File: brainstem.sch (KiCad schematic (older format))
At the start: 2 parts

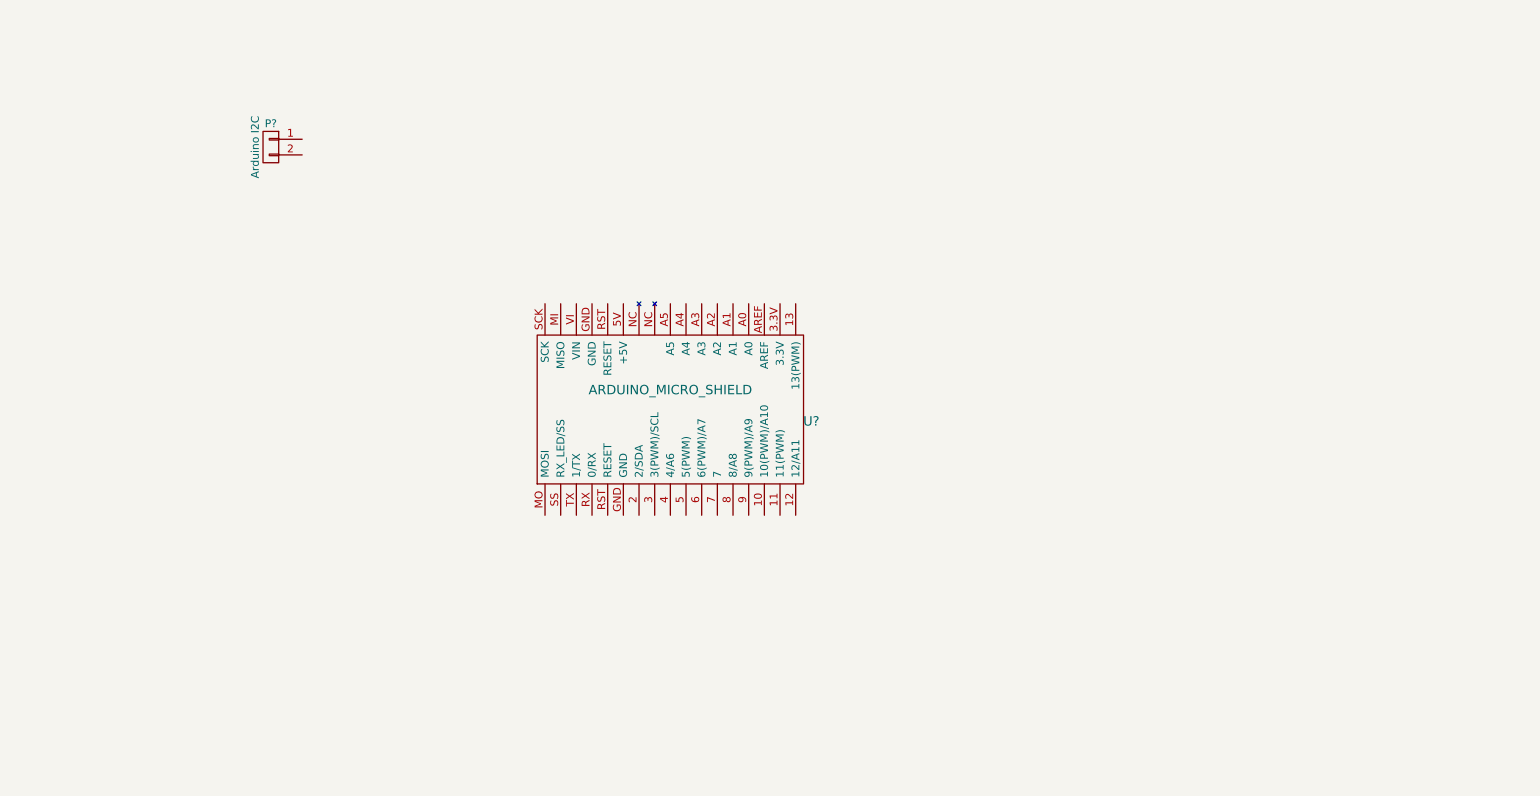
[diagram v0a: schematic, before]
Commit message: Messing around w/ kicad
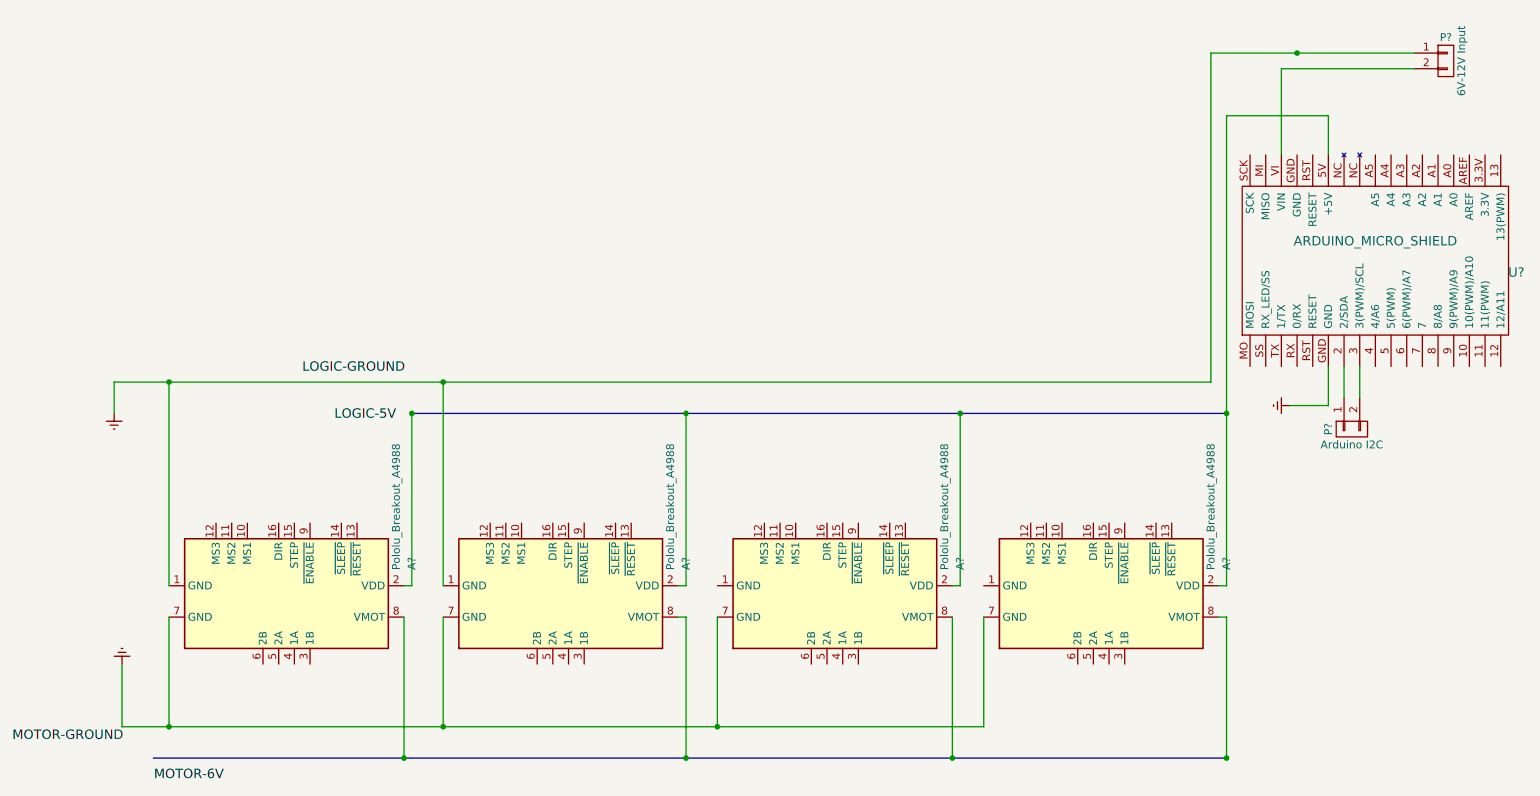
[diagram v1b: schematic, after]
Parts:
- added A? (x4): Pololu_Breakout_A4988, Module:Pololu_Breakout-16_15.2x20.3mm, symbol Pololu_Breakout_A4988
- added P?: 6V-12V Input, symbol CONN_01X02
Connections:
- net at P?.1 (P1): now also U?.2 (2/SDA)
- net at P?.2 (P2): now also U?.3 (3(PWM)/SCL)
- net at U?.5V (+5V): now also A?.2 (VDD)
- net Earth: now reaches U?.GND
- net Earth: now also A?.1 (GND), A?.1 (GND), A?.7 (GND), A?.7 (GND), A?.7 (GND), A?.7 (GND), P?.1 (P1)
- net at U?.VI (VIN): now also P?.2 (P2)
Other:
- moved on the sheet: P?, U?
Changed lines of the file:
@@
 LIBS:valves
 LIBS:arduino_micro_shield
+LIBS:Driver_Motor
 LIBS:brainstem-cache
 EELAYER 25 0
@@
 L CONN_01X02 P?
 U 1 1 5B0387E6
-P 2250 1700
-F 0 "P?" H 2250 1850 50  0000 C CNN
-F 1 "Arduino I2C" V 2350 1700 50  0000 C CNN
-F 2 "" H 2250 1700 50  0000 C CNN
-F 3 "" H 2250 1700 50  0000 C CNN
-	1    2250 1700
-	-1   0    0    -1
+P 9150 3500
+F 0 "P?" H 9150 3650 50  0000 C CNN
+F 1 "Arduino I2C" V 9250 3500 50  0000 C CNN
+F 2 "" H 9150 3500 50  0000 C CNN
+F 3 "" H 9150 3500 50  0000 C CNN
+	1    9150 3500
+	0    -1   1    0
 $EndComp
 $Comp
 L ARDUINO_MICRO_SHIELD U?
 U 1 1 5B038D80
-P 3950 3850
-F 0 "U?" H 5700 4250 60  0000 C CNN
-F 1 "ARDUINO_MICRO_SHIELD" H 4800 4450 60  0000 C CNN
-F 2 "" H 4350 3800 60  0000 C CNN
-F 3 "" H 4350 3800 60  0000 C CNN
-	1    3950 3850
+P 8450 2900
+F 0 "U?" H 10200 3300 60  0000 C CNN
+F 1 "ARDUINO_MICRO_SHIELD" H 9300 3500 60  0000 C CNN
+F 2 "" H 8850 2850 60  0000 C CNN
+F 3 "" H 8850 2850 60  0000 C CNN
+	1    8450 2900
 	1    0    0    -1
 $EndComp
+$Comp
+L CONN_01X02 P?
+U 1 1 5B03940A
+P 9750 1150
+F 0 "P?" H 9750 1300 50  0000 C CNN
+F 1 "6V-12V Input" V 9850 1150 50  0000 C CNN
+F 2 "" H 9750 1150 50  0000 C CNN
+F 3 "" H 9750 1150 50  0000 C CNN
+	1    9750 1150
+	1    0    0    -1
+$EndComp
+$Comp
+L Earth #PWR?
+U 1 1 5B039983
+P 8750 3350
+F 0 "#PWR?" H 8750 3100 50  0001 C CNN
+F 1 "Earth" H 8750 3200 50  0001 C CNN
+F 2 "" H 8750 3350 50  0000 C CNN
+F 3 "" H 8750 3350 50  0000 C CNN
+	1    8750 3350
+	0    1    1    0
+$EndComp
+$Comp
+L Pololu_Breakout_A4988 A?
+U 1 1 5B039B57
+P 5900 4500
+F 0 "A?" H 5800 5250 50  0000 R CNN
+F 1 "Pololu_Breakout_A4988" H 5800 5150 50  0000 R CNN
+F 2 "Module:Pololu_Breakout-16_15.2x20.3mm" H 6175 3750 50  0001 L CNN
+F 3 "" H 6000 4200 50  0001 C CNN
+	1    5900 4500
+	0    1    1    0
+$EndComp
+$Comp
+L Pololu_Breakout_A4988 A?
+U 1 1 5B039C62
+P 4150 4500
+F 0 "A?" H 4050 5250 50  0000 R CNN
+F 1 "Pololu_Breakout_A4988" H 4050 5150 50  0000 R CNN
+F 2 "Module:Pololu_Breakout-16_15.2x20.3mm" H 4425 3750 50  0001 L CNN
+F 3 "" H 4250 4200 50  0001 C CNN
+	1    4150 4500
+	0    1    1    0
+$EndComp
+$Comp
+L Pololu_Breakout_A4988 A?
+U 1 1 5B039CE5
+P 2400 4500
+F 0 "A?" H 2300 5250 50  0000 R CNN
+F 1 "Pololu_Breakout_A4988" H 2300 5150 50  0000 R CNN
+F 2 "Module:Pololu_Breakout-16_15.2x20.3mm" H 2675 3750 50  0001 L CNN
+F 3 "" H 2500 4200 50  0001 C CNN
+	1    2400 4500
+	0    1    1    0
+$EndComp
+$Comp
+L Pololu_Breakout_A4988 A?
+U 1 1 5B03A05C
+P 7600 4500
+F 0 "A?" H 7500 5250 50  0000 R CNN
+F 1 "Pololu_Breakout_A4988" H 7500 5150 50  0000 R CNN
+F 2 "Module:Pololu_Breakout-16_15.2x20.3mm" H 7875 3750 50  0001 L CNN
+F 3 "" H 7700 4200 50  0001 C CNN
+	1    7600 4500
+	0    1    1    0
+$EndComp
+Text Label 1950 5750 2    60   ~ 0
+MOTOR-6V
+Text Label 3050 3450 2    60   ~ 0
+LOGIC-5V
+Text Label 2450 3150 0    60   ~ 0
+LOGIC-GROUND
+Wire Wire Line
+	9000 3350 9000 3100
+Connection ~ 8800 1100
+Wire Wire Line
+	8700 1750 8700 1200
+Wire Wire Line
+	8700 1200 9550 1200
+Wire Wire Line
+	8250 1100 8800 1100
+Wire Wire Line
+	8800 1100 9550 1100
+Wire Wire Line
+	8750 3350 9000 3350
+Wire Wire Line
+	9100 3100 9100 3300
+Wire Wire Line
+	9200 3300 9200 3100
+Wire Bus Line
+	1500 5600 3100 5600
+Wire Bus Line
+	3100 5600 4900 5600
+Wire Bus Line
+	4900 5600 6600 5600
+Wire Bus Line
+	6600 5600 8350 5600
+Connection ~ 8350 5600
+Wire Bus Line
+	3150 3400 4900 3400
+Wire Bus Line
+	4900 3400 6650 3400
+Wire Bus Line
+	6650 3400 8350 3400
+Connection ~ 8350 3400
+Wire Wire Line
+	9000 1750 9000 1500
+Wire Wire Line
+	9000 1500 8350 1500
+Wire Wire Line
+	8350 1500 8350 3400
+Wire Wire Line
+	8350 3400 8350 4500
+Wire Wire Line
+	1250 3200 1600 3200
+Wire Wire Line
+	1600 3200 3350 3200
+Wire Wire Line
+	3350 3200 8250 3200
+Wire Wire Line
+	8250 3200 8250 1100
+Wire Wire Line
+	3350 4500 3350 3200
+Connection ~ 3350 3200
+Wire Wire Line
+	1600 4500 1600 3200
+Connection ~ 1600 3200
+Connection ~ 3150 3400
+Wire Wire Line
+	3150 3400 3150 4500
+Wire Wire Line
+	3150 4500 3100 4500
+Connection ~ 4900 3400
+Wire Wire Line
+	4900 3400 4900 4500
+Wire Wire Line
+	4900 4500 4850 4500
+Connection ~ 6650 3400
+Wire Wire Line
+	6650 3400 6650 4500
+Wire Wire Line
+	6650 4500 6600 4500
+Wire Wire Line
+	8350 4500 8300 4500
+Wire Wire Line
+	8350 3400 8350 3400
+Connection ~ 3100 5600
+Wire Wire Line
+	3100 4700 3100 4700
+Wire Wire Line
+	3100 4700 3100 5600
+Connection ~ 4900 5600
+Wire Wire Line
+	4900 5600 4900 4700
+Wire Wire Line
+	4900 4700 4850 4700
+Connection ~ 6600 5600
+Wire Wire Line
+	6600 4700 6600 5600
+Wire Wire Line
+	8300 4700 8350 4700
+Wire Wire Line
+	8350 4700 8350 5600
+$Comp
+L Earth #PWR?
+U 1 1 5B03ADA8
+P 1250 3400
+F 0 "#PWR?" H 1250 3150 50  0001 C CNN
+F 1 "Earth" H 1250 3250 50  0001 C CNN
+F 2 "" H 1250 3400 50  0000 C CNN
+F 3 "" H 1250 3400 50  0000 C CNN
+	1    1250 3400
+	1    0    0    -1
+$EndComp
+Wire Wire Line
+	1250 3400 1250 3200
+Text Label 600  5500 0    60   ~ 0
+MOTOR-GROUND
+$Comp
+L Earth #PWR?
+U 1 1 5B03AEB4
+P 1300 5000
+F 0 "#PWR?" H 1300 4750 50  0001 C CNN
+F 1 "Earth" H 1300 4850 50  0001 C CNN
+F 2 "" H 1300 5000 50  0000 C CNN
+F 3 "" H 1300 5000 50  0000 C CNN
+	1    1300 5000
+	-1   0    0    1
+$EndComp
+Wire Wire Line
+	6800 5400 6800 4700
+Wire Wire Line
+	1300 5400 1600 5400
+Wire Wire Line
+	1600 5400 3350 5400
+Wire Wire Line
+	3350 5400 5100 5400
+Wire Wire Line
+	5100 5400 6800 5400
+Wire Wire Line
+	1300 5400 1300 5000
+Wire Wire Line
+	5100 4700 5100 5400
+Connection ~ 5100 5400
+Wire Wire Line
+	3350 4700 3350 5400
+Connection ~ 3350 5400
+Wire Wire Line
+	1600 4700 1600 5400
+Connection ~ 1600 5400
 $EndSCHEMATC
